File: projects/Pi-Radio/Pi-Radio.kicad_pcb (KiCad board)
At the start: 2 copper layers, 65 x 56 mm, 24 parts, among them J1 Data, J8 Power, SW1 Left, SW2 Time, SW3 Up, SW4 Special, SW5 PlayStop, SW6 Down, SW7 Right

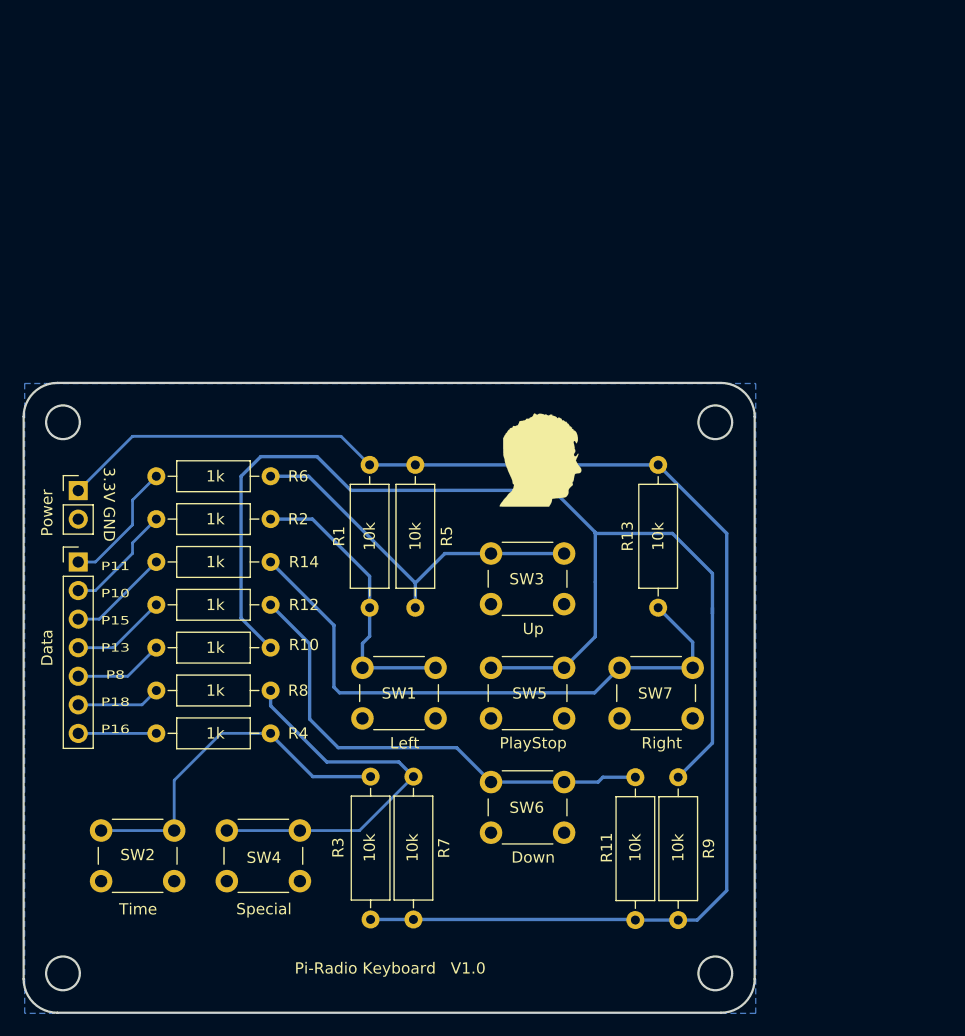
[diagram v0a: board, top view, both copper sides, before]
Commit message: updates
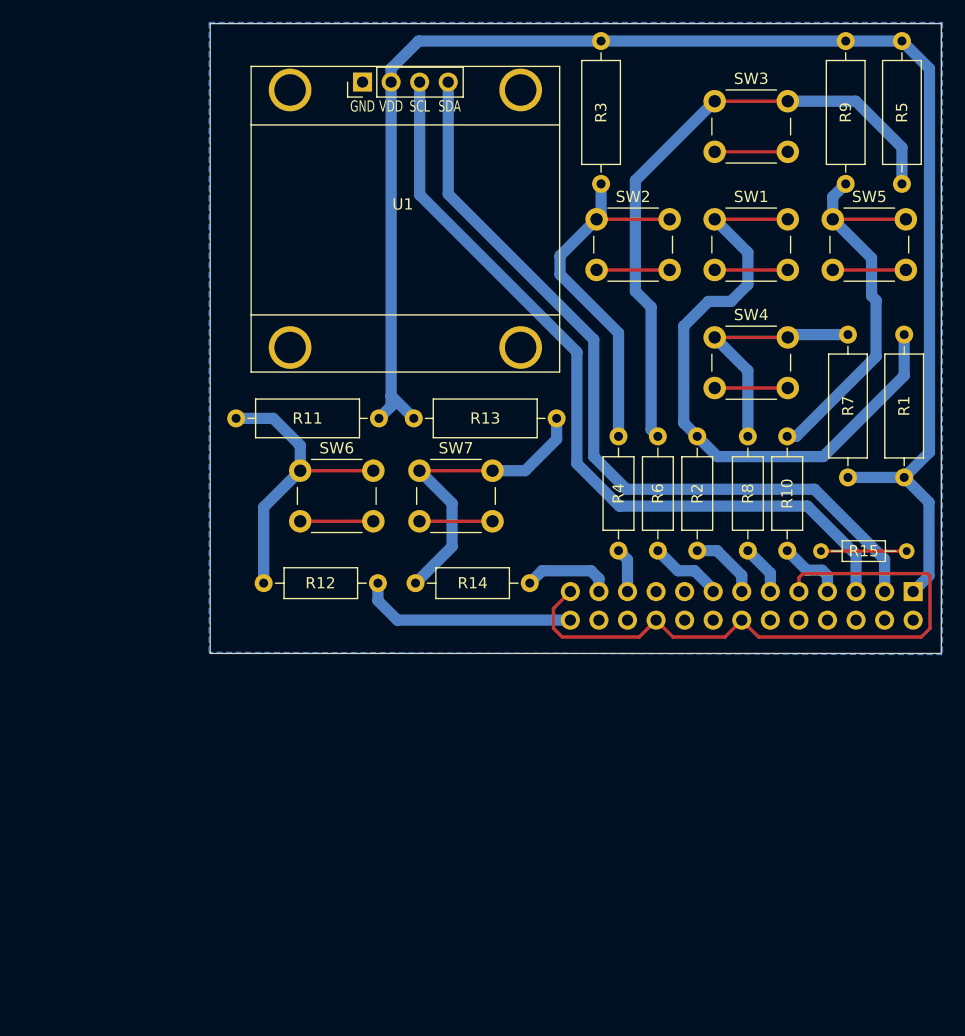
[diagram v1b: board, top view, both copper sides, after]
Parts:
- removed J8: Power, Connector_PinHeader_2.54mm:PinHeader_1x02_P2.54mm_Vertical
- removed Silvan Logo: Logo, Logos:silvan_logo_10mm
- added R15: 0, Resistor_THT:R_Axial_DIN0204_L3.6mm_D1.6mm_P7.62mm_Horizontal, F.Cu at (171.8, 114.4)
- added U1: Display_OLED_I2C_0.96, OLED:Display_128x64_096_I2C, F.Cu at (134.8, 93.4)
- J1: value Data -> Conn_02x13_Odd_Even; footprint Connector_PinHeader_2.54mm:PinHeader_1x07_P2.54mm_Vertical -> Connector_PinSocket_2.54mm:PinSocket_2x13_P2.54mm_Vertical; moved to B.Cu
- SW1: value Left -> Button_PlayStop; footprint Button_Switch_THT:SW_PUSH_6mm_H5mm -> Button_Switch_THT:SW_PUSH_6mm
- SW2: value Time -> Button_Left; footprint Button_Switch_THT:SW_PUSH_6mm_H5mm -> Button_Switch_THT:SW_PUSH_6mm
- SW3: value Up -> Button_Up; footprint Button_Switch_THT:SW_PUSH_6mm_H5mm -> Button_Switch_THT:SW_PUSH_6mm
- SW4: value Special -> Button_Down; footprint Button_Switch_THT:SW_PUSH_6mm_H5mm -> Button_Switch_THT:SW_PUSH_6mm
- SW5: value PlayStop -> Button_Right; footprint Button_Switch_THT:SW_PUSH_6mm_H5mm -> Button_Switch_THT:SW_PUSH_6mm
- SW6: value Down -> Button_Time; footprint Button_Switch_THT:SW_PUSH_6mm_H5mm -> Button_Switch_THT:SW_PUSH_6mm
- SW7: value Right -> Button_Special; footprint Button_Switch_THT:SW_PUSH_6mm_H5mm -> Button_Switch_THT:SW_PUSH_6mm
- moved J1 74.3 mm to (180.0, 118.0), turned to 90 degrees
- moved SW2 70.0 mm to (151.8, 84.9)
- moved SW4 61.7 mm to (162.3, 95.4)
- moved R5 57.4 mm to (179.0, 81.8)
- moved R3 56.5 mm to (152.2, 81.8), turned to 90 degrees
- moved R7 55.1 mm to (174.2, 95.2)
- moved R9 54.8 mm to (174.0, 81.8), turned to 90 degrees
- moved R1 53.4 mm to (179.2, 95.2), turned to 270 degrees
- moved SW1 50.7 mm to (162.3, 84.9)
- moved SW5 50.1 mm to (172.8, 84.9)
- moved R10 49.6 mm to (168.8, 104.2), turned to 270 degrees
- moved R8 48.1 mm to (165.3, 104.2), turned to 270 degrees
- moved R11 47.7 mm to (119.8, 102.6), turned to 0 degrees
- moved SW3 44.9 mm to (162.3, 74.4)
- moved R4 40.7 mm to (153.8, 104.2), turned to 270 degrees
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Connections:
- J1 pad 1: Pin11 -> +3V3
- J1 pad 2: Pin10 -> (no net)
- J1 pad 3: Pin15 -> SDA
- J1 pad 4: Pin13 -> (no net)
- J1 pad 5: Pin8 -> SCL
- J1 pad 6: Pin18 -> (no net)
- J1 pad 7: Pin16 -> Pin07
- R10 pad 2: Pin8 -> Pin07
- R12 pad 2: Pin13 -> Pin26
- R14 pad 2: Pin15 -> Pin23
- R2 pad 2: Pin10 -> Pin13
- R4 pad 2: Pin16 -> Pin21
- R6 pad 2: Pin11 -> Pin15
- R8 pad 2: Pin18 -> Pin11
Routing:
- net GND: track 0.00 -> 111.4 mm
- net SDA: track 0.00 -> 71.2 mm
- net SCL: track 0.00 -> 71.2 mm
- net Net-(R10-Pad1): track 102.8 -> 34.8 mm
- net Net-(R1-Pad1): track 25.8 -> 56.8 mm
- net Net-(R13-Pad1): track 53.1 -> 27.8 mm
- net Net-(R5-Pad1): track 33.3 -> 55.1 mm
- net Pin26: track 0.00 -> 19.4 mm
- net Net-(R11-Pad1): track 43.7 -> 26.8 mm
- net Net-(R7-Pad1): track 35.2 -> 22.0 mm
- net +3V3: track 127.8 -> 138.2 mm
- net Pin10: track 10.1 -> 0.00 mm
- net Pin23: track 0.00 -> 8.04 mm
- net Pin8: track 8.00 -> 0.00 mm
- net Pin18: track 7.84 -> 0.00 mm
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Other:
- outline, holes or cut-outs redrawn
- net class Default: clearance 0.2 -> 0.5; trace_width 0.25 -> 1
- rule trace_clearance: 0.2 -> 0.5
- board text removed: "3.3V"
- board text removed: "GND"
- board text removed: "P11 P10 P15 P13 P8 P18 P16"
- board text removed: "Pi-Radio Keyboard V1.0"
